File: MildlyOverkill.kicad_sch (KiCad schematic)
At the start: 72 parts, among them J1 USB_C_Receptacle_USB2.0_16P, J10 Conn_01x07_Pin, J11 Conn_01x08_Pin, J2 Screw_Terminal_01x02, J3 Motors, J4 IO, J5 Conn_01x04_Pin, J6 Conn_01x04_MountingPin, J7 GND, J8 VCC, J9 Analog, M1 Fan_4pin, Q1 Q_PMOS_GDS, U1 ESP32-S3-WROOM-1, U2 MCP3208, U3 LD1117S33TR_SOT223, U5 USBLC6-2P6, U6 TPS62932

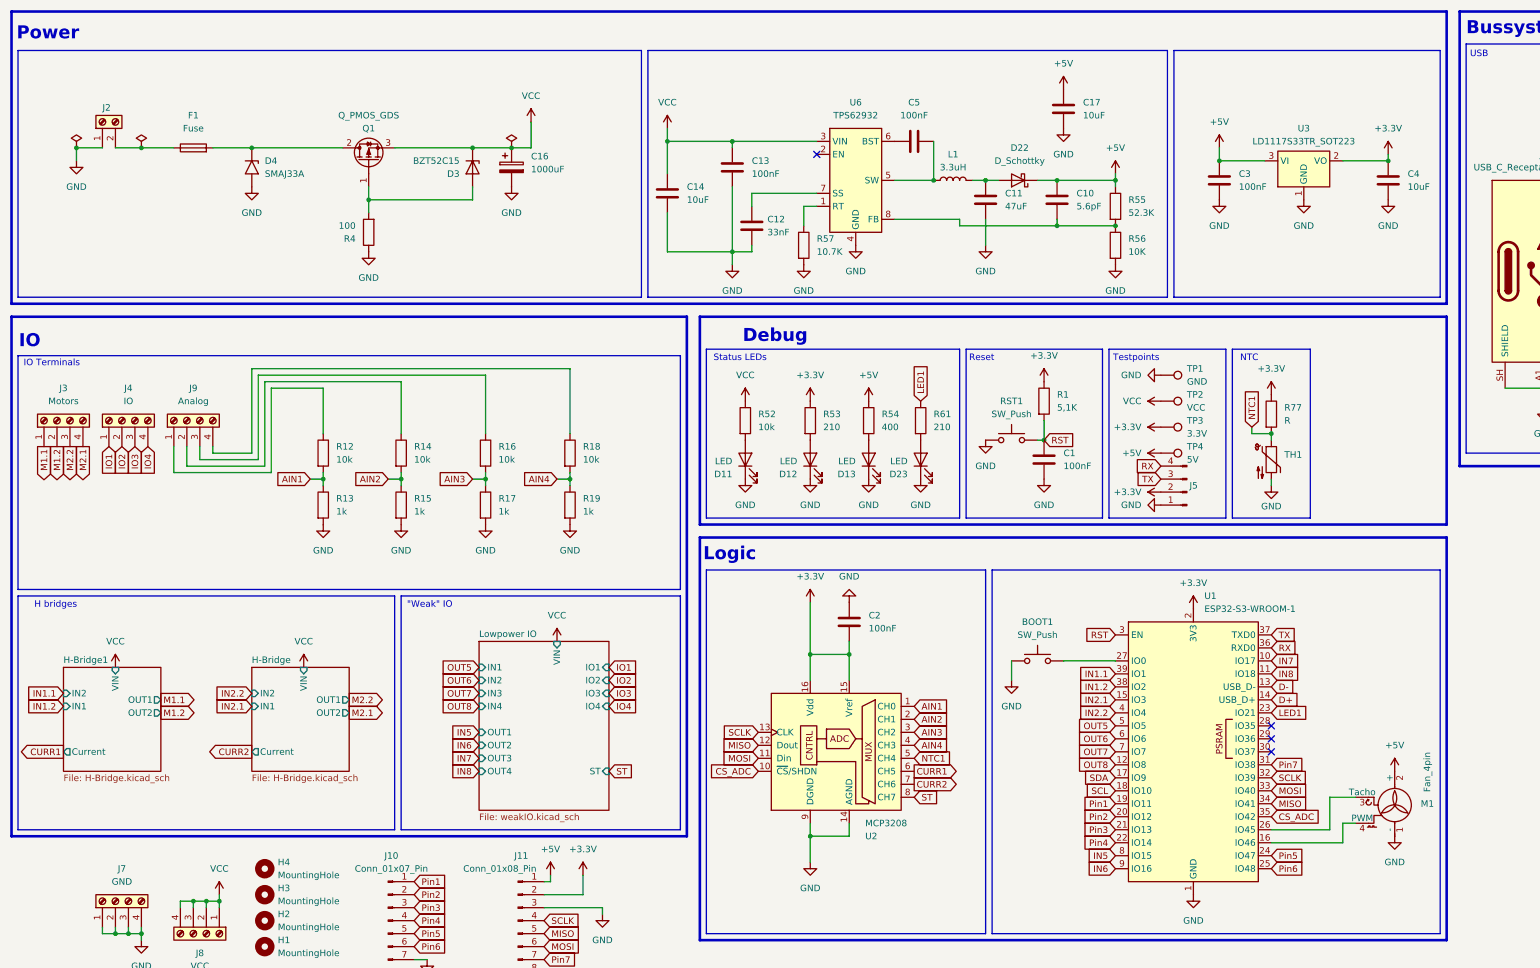
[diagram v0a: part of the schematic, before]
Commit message: DONE!!!
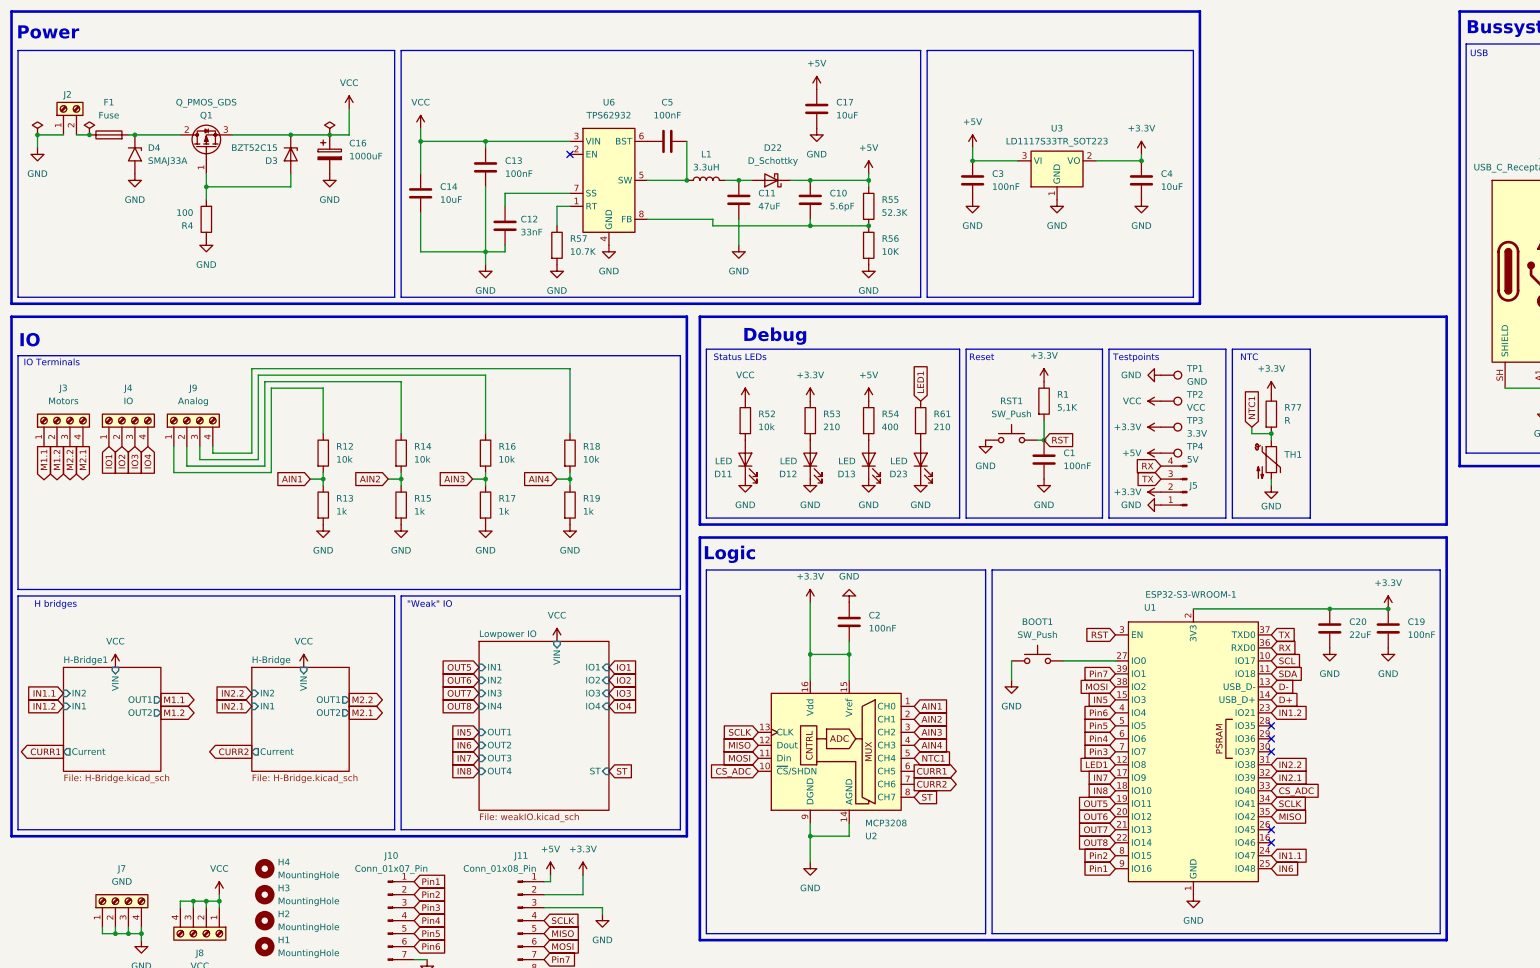
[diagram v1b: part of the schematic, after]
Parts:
- removed M1: Fan_4pin, Connector:FanPinHeader_1x04_P2.54mm_Vertical, symbol Motor:Fan_4pin
- added C19: 100nF, Capacitor_SMD:C_0603_1608Metric, symbol Device:C
- added C20: 22uF, Capacitor_SMD:C_0603_1608Metric, symbol Device:C
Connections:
- net +3.3V: now also C19.1, C20.1
- net CS_ADC: now also U1.33 (IO40); no longer U1.35 (IO42)
- net GND: now also C19.2, C20.2
- net IN1.1: now also U1.24 (IO47); no longer U1.39 (IO1)
- net IN1.2: now also U1.23 (IO21); no longer U1.38 (IO2)
- net IN2.1: now also U1.32 (IO39); no longer U1.15 (IO3)
- net IN2.2: now also U1.31 (IO38); no longer U1.4 (IO4)
- net IN5: now also U1.15 (IO3); no longer U1.8 (IO15)
- net IN6: now also U1.25 (IO48); no longer U1.9 (IO16)
- net IN7: now also U1.17 (IO9); no longer U1.10 (IO17)
- net IN8: now also U1.18 (IO10); no longer U1.11 (IO18)
- net LED1: now also U1.12 (IO8); no longer U1.23 (IO21)
- net MISO: now also U1.35 (IO42); no longer U1.34 (IO41)
- net MOSI: now also U1.38 (IO2); no longer U1.33 (IO40)
- net OUT5: now also U1.19 (IO11); no longer U1.5 (IO5)
- net OUT6: now also U1.20 (IO12); no longer U1.6 (IO6)
- net OUT7: now also U1.21 (IO13); no longer U1.7 (IO7)
- net OUT8: now also U1.22 (IO14); no longer U1.12 (IO8)
- net Pin1: now also U1.9 (IO16); no longer U1.19 (IO11)
- net Pin2: now also U1.8 (IO15); no longer U1.20 (IO12)
- net Pin3: now also U1.7 (IO7); no longer U1.21 (IO13)
- net Pin4: now also U1.6 (IO6); no longer U1.22 (IO14)
- net Pin5: now also U1.5 (IO5); no longer U1.24 (IO47)
- net Pin6: now also U1.4 (IO4); no longer U1.25 (IO48)
- net Pin7: now also U1.39 (IO1); no longer U1.31 (IO38)
- net SCL: now also U1.10 (IO17); no longer U1.18 (IO10)
- net SCLK: now also U1.34 (IO41); no longer U1.32 (IO39)
- net SDA: now also U1.11 (IO18); no longer U1.17 (IO9)
- no-connect marks 6 -> 8
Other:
- moved on the sheet: C10, C11, C12, C13, C14, C16, C17, C3, C4, C5, D22, D3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
